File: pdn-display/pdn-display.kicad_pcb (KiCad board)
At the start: 2 copper layers, 86.4 x 66 mm, 42 parts, among them CN1 PH-3AW_C722773, CN2 PH-6AW_C722785, U5 Display

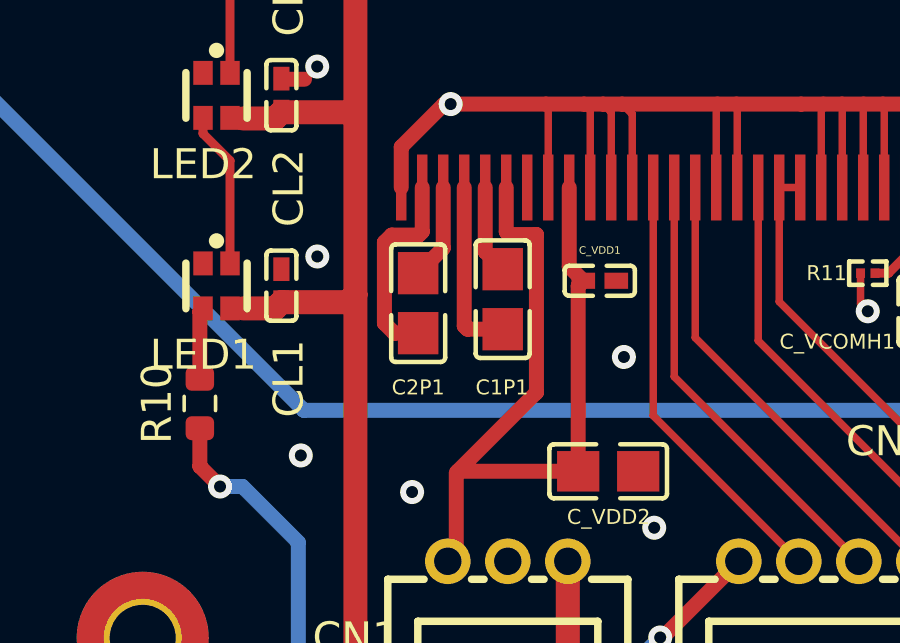
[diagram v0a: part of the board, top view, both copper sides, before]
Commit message: 2025 Production Files.
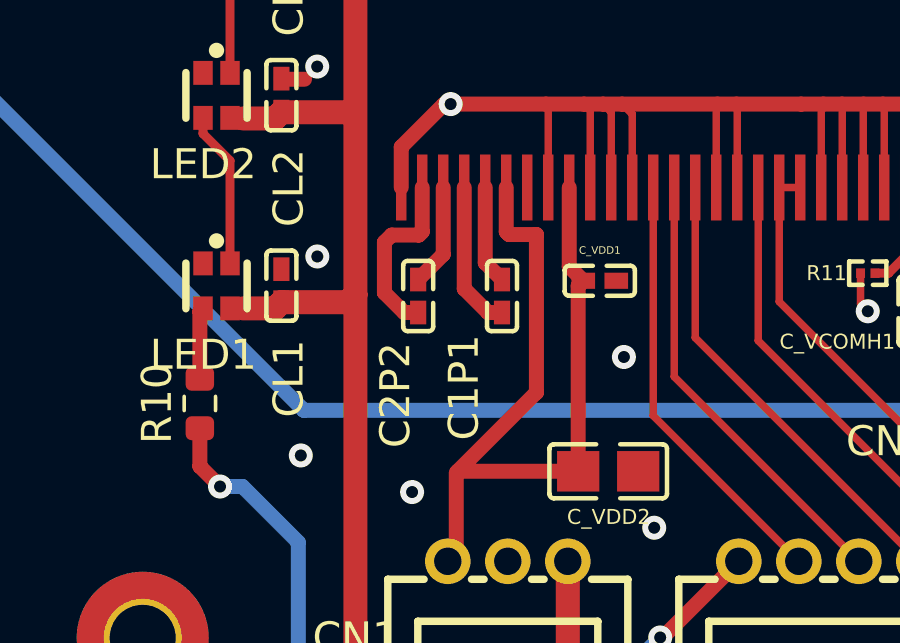
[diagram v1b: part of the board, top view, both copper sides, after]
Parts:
- removed C2P1: 1uF, global:C0805
- added C2P2: 1uF, global:C0402, F.Cu at (77.0, 74.7)
- C1P1: footprint global:C0805 -> global:C0402
- moved C1P1 0.11 mm to (79.8, 74.7)
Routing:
- net Net-(U5-C1P): track 5.94 -> 4.96 mm
- net Net-(U5-C2P): track 6.84 -> 5.96 mm
